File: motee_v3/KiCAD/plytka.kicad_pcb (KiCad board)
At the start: 2 copper layers, 58 parts, among them J1 SN65HVD3082EDGK, U1 STM32F103, U10 pad, U11 pad, U12 pad, U13 pad, U14 pad, U15 pad, U16 pad, U17 pad, U18 pad, U19 pad, U2 DRV8801, U20 pad, U21 pad, U22 pad, U23 pad, U24 pad, U25 pad, U26 pad, U27 pad, U28 pad, U29 pad, U3 TLE4946-2K, U30 pad, U31 pad, U32 pad, U33 pad, U34 pad, U4 TLE4946-2K, U5 pad_round, U6 pad_round, U7 micro-usb, U8 LP38693, U9 LP38693

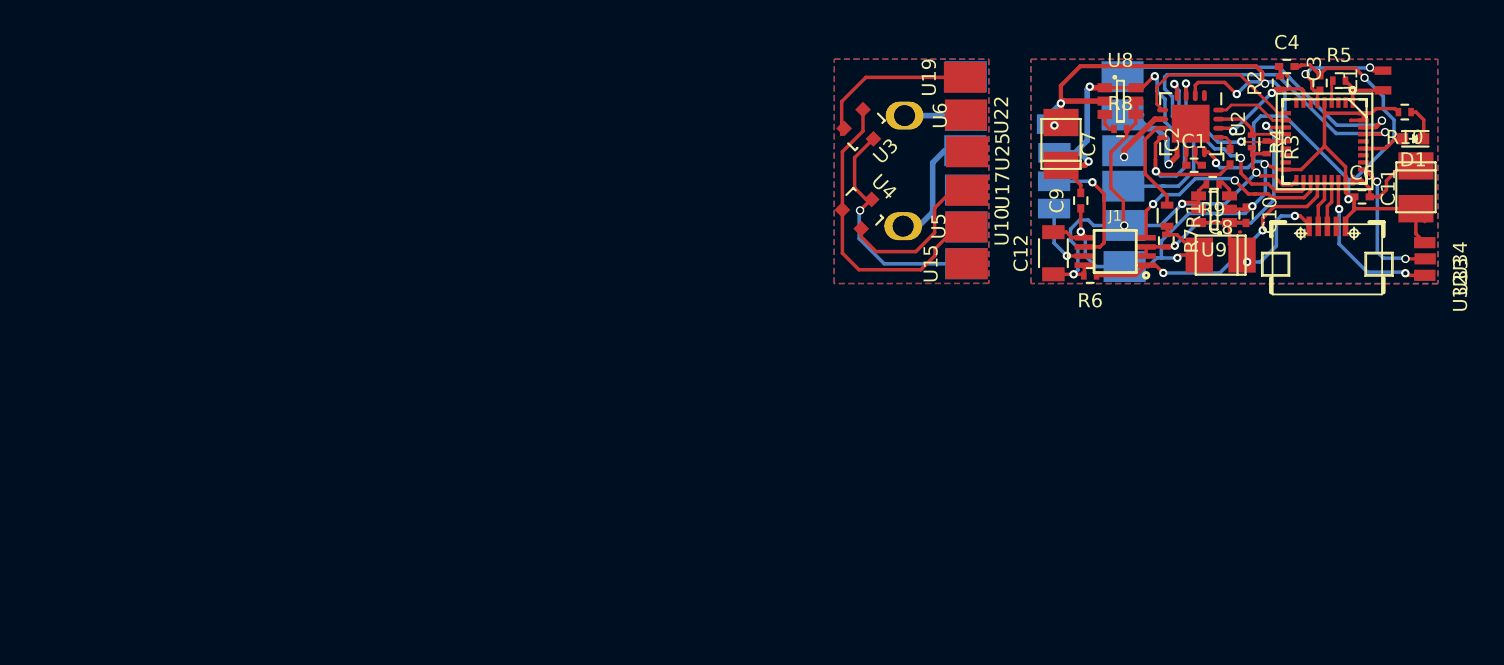
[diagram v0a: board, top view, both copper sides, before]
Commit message: bug fixes
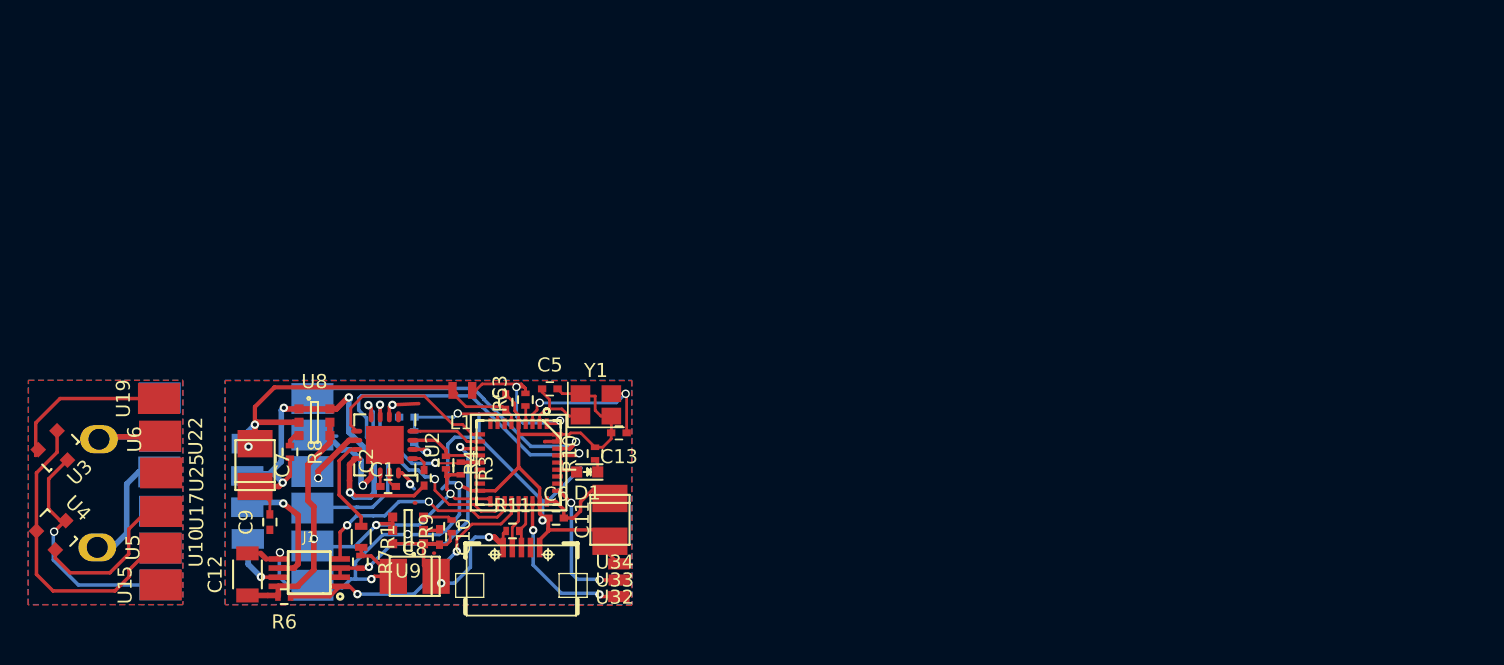
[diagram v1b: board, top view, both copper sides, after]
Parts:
- added C13: 22pF, Capacitors_SMD:C_0402, F.Cu at (58.7, 178.6)
- added C5: 22pF, Capacitors_SMD:C_0402, F.Cu at (53.7, 175.5)
- added R11: 1k, Resistors_SMD:R_0402, F.Cu at (51.1, 185.6)
- added Y1: Crystal_GND24, Crystals:Crystal_SMD_SeikoEpson_FA238-4pin_3.2x2.5mm, F.Cu at (57.0, 176.6)
- C4, R2: moved to B.Cu
- U8, U9: footprint TO_SOT_Packages_SMD:SOT-23-6 -> LP38693:SOT-23-6
- moved L1 69.2 mm to (47.5, 175.6), turned to 180 degrees
- moved C4 67.5 mm to (43.5, 177.5), turned to 180 degrees
- moved R2 66.6 mm to (44.1, 178.9)
- moved R8 63.5 mm to (35.2, 180.0), turned to 270 degrees
- moved D1 63.4 mm to (56.4, 181.4)
- moved R10 62.6 mm to (57.0, 180.1), turned to 90 degrees
- moved C3 62.3 mm to (50.6, 176.4)
- moved R5 62.3 mm to (52.0, 176.3), turned to 90 degrees
- moved U12 62.2 mm to (36.8, 186.7)
- moved U14 62.1 mm to (36.8, 189.5)
- moved U16 62.1 mm to (36.8, 184.0)
- moved C9 62.1 mm to (33.8, 185.0)
- moved U27 62.1 mm to (36.8, 181.4)
- moved C11 62.1 mm to (58.0, 184.8)
- moved U20 62.1 mm to (36.8, 176.2)
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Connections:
- R8 pad 2: +3V3 -> +8V
- R9 pad 1: Net-(R9-Pad1) -> VBUS
- R9 pad 2: +3V3 -> Net-(R9-Pad2)
- U1 pad 2: (no net) -> Net-(C5-Pad1)
- U1 pad 3: (no net) -> Net-(C13-Pad1)
- U9 pad 3: Net-(R9-Pad1) -> Net-(R9-Pad2)
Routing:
- net GND: track 151.3 -> 122.0 mm, vias 12 -> 9
- net Net-(C3-Pad1): track 8.44 -> 23.0 mm, vias 2 -> 1
- net Net-(C13-Pad1): track 0.00 -> 12.2 mm, vias 0 -> 2
- net Net-(R2-Pad1): track 8.45 -> 2.30 mm, vias 2 -> 1
- net ADC: track 1.78 -> 7.65 mm, vias 0 -> 1
- net Net-(C5-Pad1): track 0.00 -> 5.55 mm
- net OUT2: track 12.7 -> 17.1 mm
- net +3V3: track 75.6 -> 79.4 mm, vias 4 -> 5
- net +8V: track 38.0 -> 41.4 mm
- net VBUS: track 15.2 -> 18.1 mm
- net Net-(R9-Pad2): track 0.00 -> 2.09 mm
- net Net-(D1-Pad1): track 2.48 -> 0.94 mm
- net Net-(D1-Pad2): track 3.85 -> 2.34 mm
- net Net-(R9-Pad1): track 1.34 -> 0.00 mm
